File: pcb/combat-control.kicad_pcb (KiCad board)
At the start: 4 copper layers, 59 x 30.2 mm, 130 parts, among them J1 Conn_01x01_Pin, J2 Conn_01x01_Pin, J3 Conn_01x01_Pin, J4 Conn_01x01_Pin, J5 Conn_01x01_Pin, J6 Conn_01x01_Pin, J7 Conn_01x01_Pin, J8 Conn_01x01_Pin, Q1 AON7544, Q10 AON7544, Q11 AON7544, Q12 AON7544, Q2 AON7544, Q3 AON7544, Q4 AON7544, Q5 AON7544, Q6 AON7544, Q7 AON7544, Q8 AON7544, Q9 AON7544, U1 ICM-42688-P, U10 TPHR8504PL, U11 TPHR8504PL, U12 TPHR8504PL, U2 ESP32-S3, U3 DRV8328B, U4 DRV8328B, U5 DRV8328B, U6 ACS781xLRTR-100B, U7 TPHR8504PL, U8 TPHR8504PL, U9 TPHR8504PL, Y1 40MHz

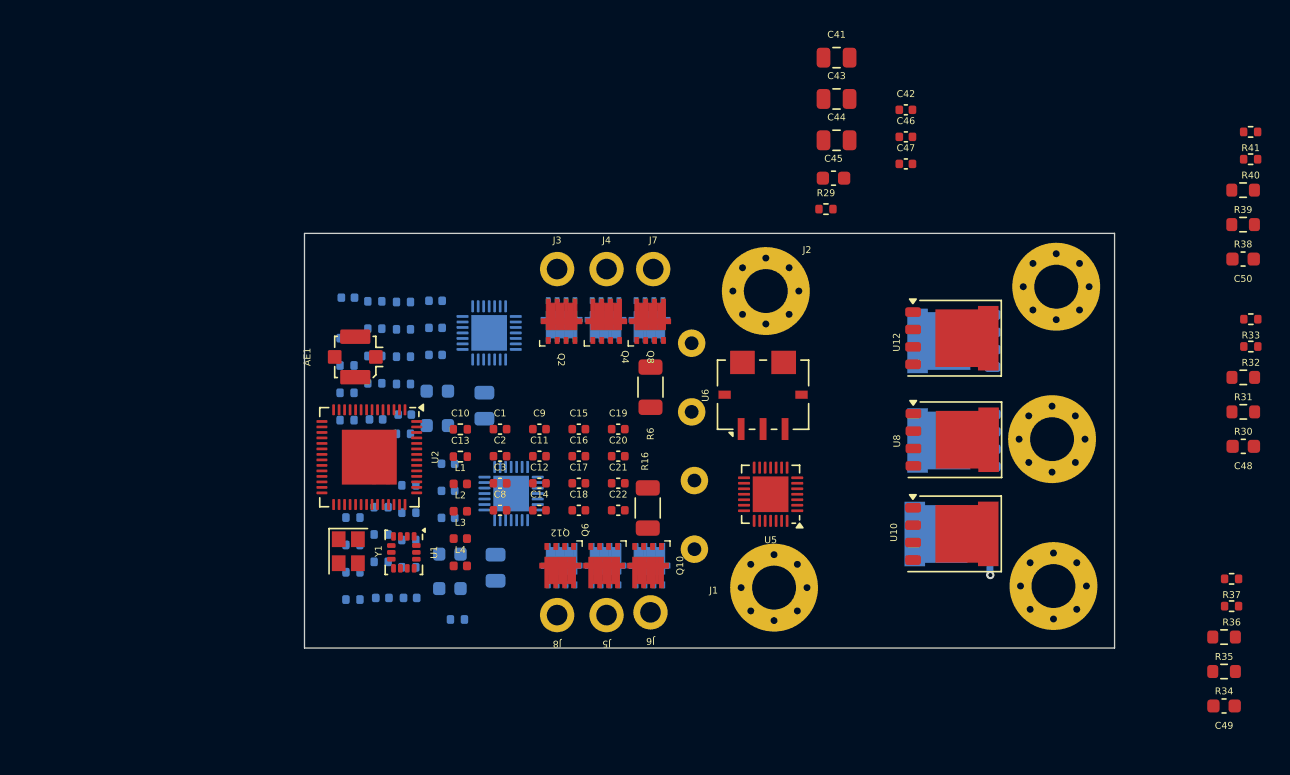
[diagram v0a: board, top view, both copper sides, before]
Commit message: Save layout
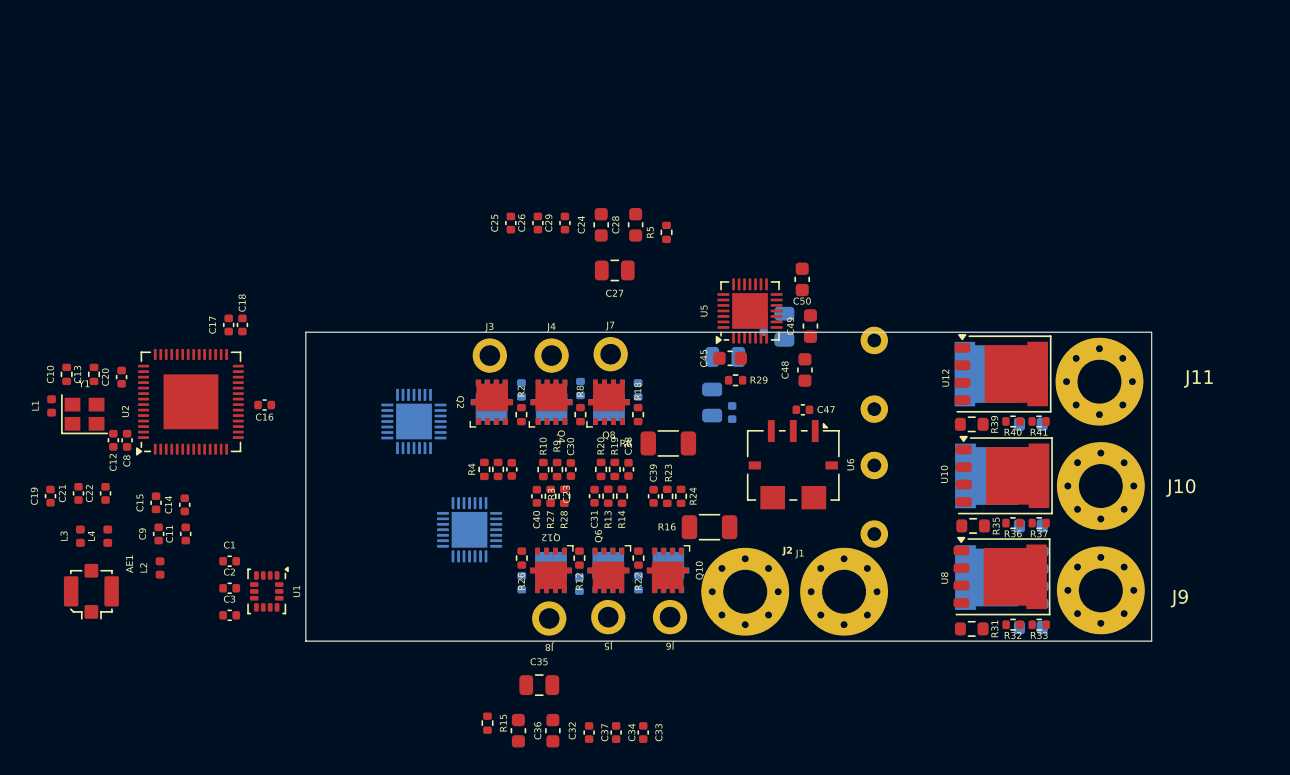
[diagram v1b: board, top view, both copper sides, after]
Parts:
- removed C6: 2m2, User_Footprints:C_D10xL16_Horizontal
- removed the J2 at (111.6, 49.6)
- removed the J2 at (132.6, 71.1)
- removed the J2 at (132.4, 60.4)
- removed the J2 at (132.8, 49.3)
- added C5: 2m2, User_Footprints:C_D10xL16_Horizontal, B.Cu at (119.5, 58.2)
- added J10: Conn_01x01_Pin, MountingHole:MountingHole_3.2mm_M3_Pad_Via, F.Cu at (136.0, 63.8)
- added J11: Conn_01x01_Pin, MountingHole:MountingHole_3.2mm_M3_Pad_Via, F.Cu at (135.9, 56.2)
- added J2: Conn_01x01_Pin, MountingHole:MountingHole_3.2mm_M3_Pad_Via, F.Cu at (110.1, 71.5)
- added J9: Conn_01x01_Pin, MountingHole:MountingHole_3.2mm_M3_Pad_Via, F.Cu at (136.0, 71.4)
- C23, C24, C25, C26, C27, C28, C29, C30, C31, C32, C33, C34, C35, C36, C37, C38, C39, C40, R10, R12, R13, R14, R15, R18, R19, R2, R20, R22, R23, R24, R26, R27, R28, R3, R4, R5, R8, R9: moved to F.Cu
- C41, C42, C43, C44, C46, R30, R34, R38: moved to B.Cu
- moved C19 41.6 mm to (59.5, 64.5), turned to 90 degrees
- moved C49 40.9 mm to (114.9, 52.1), turned to 90 degrees
- moved C21 39.3 mm to (61.5, 64.3), turned to 90 degrees
- moved C22 37.4 mm to (63.5, 64.3), turned to 90 degrees
- moved C20 36.6 mm to (64.7, 55.9), turned to 90 degrees
- moved C48 32.4 mm to (114.5, 55.4), turned to 90 degrees
- moved C50 32.1 mm to (114.3, 48.8), turned to 90 degrees
- moved C15 31.3 mm to (67.2, 65.0), turned to 90 degrees
- moved C12 31.2 mm to (64.1, 60.5), turned to 90 degrees
- moved L1 30.3 mm to (59.6, 58.0), turned to 90 degrees
- moved C10 28.9 mm to (60.7, 55.7), turned to 90 degrees
- moved C9 28.8 mm to (67.4, 67.3), turned to 90 degrees
- moved C17 28.0 mm to (72.5, 52.1), turned to 90 degrees
- moved C18 28.0 mm to (73.5, 52.1), turned to 90 degrees
- moved L3 27.7 mm to (61.7, 67.5), turned to 90 degrees
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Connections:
- C4 pad 2: GND -> /LargeMotor/LOW
- U2 pad 5: unconnected-(U2-GPIO0-Pad5) -> /IFIG
- U2 pad 51: unconnected-(U2-GPIO45-Pad51) -> /IFIG
- U6 pad 5: /LargeMotor/LOW -> GND
- U6 pad 6: GND -> /LargeMotor/LOW
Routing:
- net Net-(U9-G): track 1.10 -> 0.00 mm, vias 1 -> 0
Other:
- board size 59 x 30.2 mm -> 61.6 x 22.5 mm

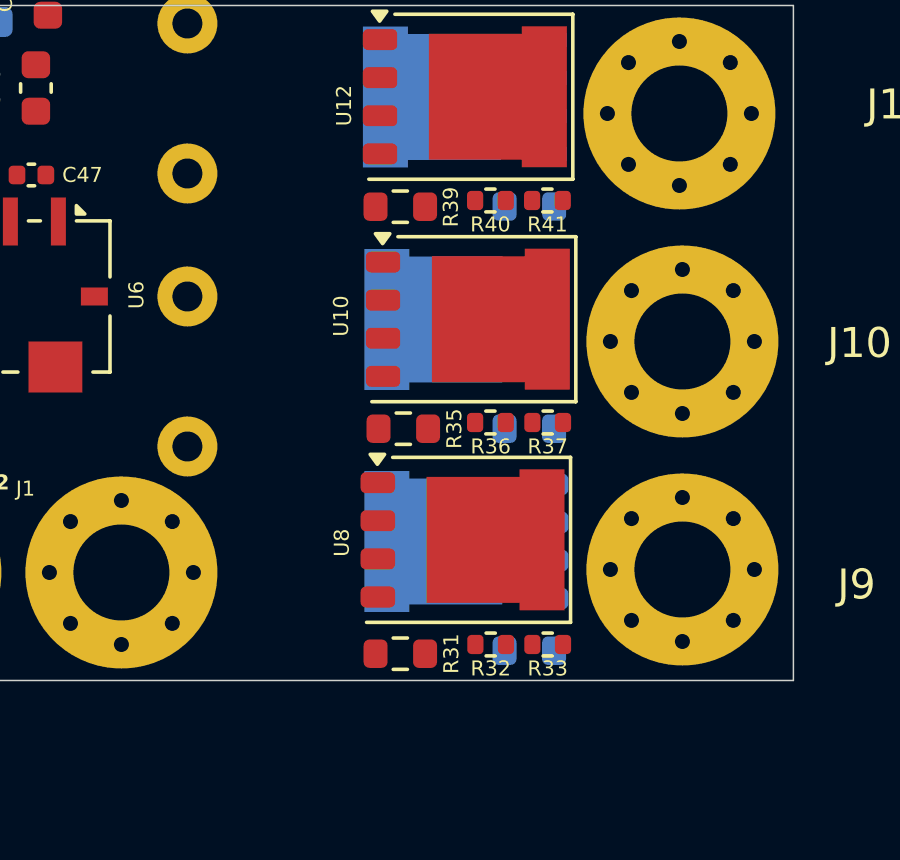
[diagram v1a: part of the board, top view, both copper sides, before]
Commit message: Save layout
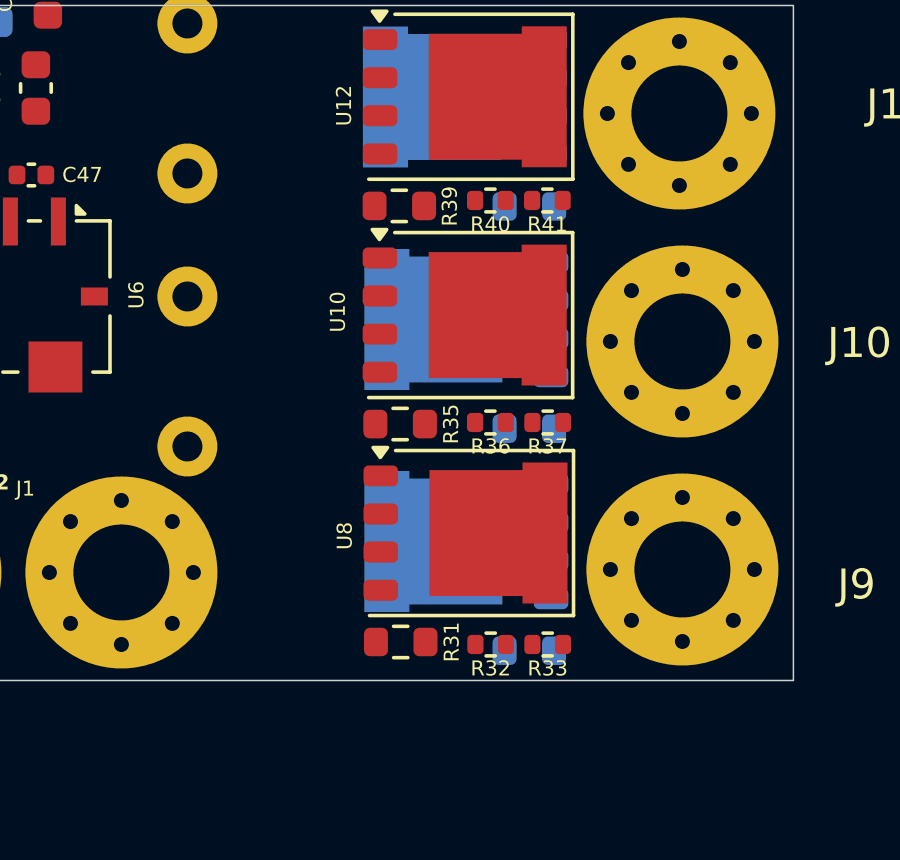
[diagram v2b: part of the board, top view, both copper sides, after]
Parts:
- moved R31 0.39 mm to (126.6, 73.8)
- moved U8 0.25 mm to (128.7, 70.2)
- moved R35 0.19 mm to (126.6, 66.6)
- moved U10 0.17 mm to (128.6, 62.9)
